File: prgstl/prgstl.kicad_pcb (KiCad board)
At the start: 2 copper layers, 76.2 x 50.8 mm, 49 parts, among them J2 STM32WORLD_BASE, Q1 S9013, U1 AMS1117-3.3``, U2 STM32F103CBTx, U3 SRV05-4, Y1 X_8MHZ

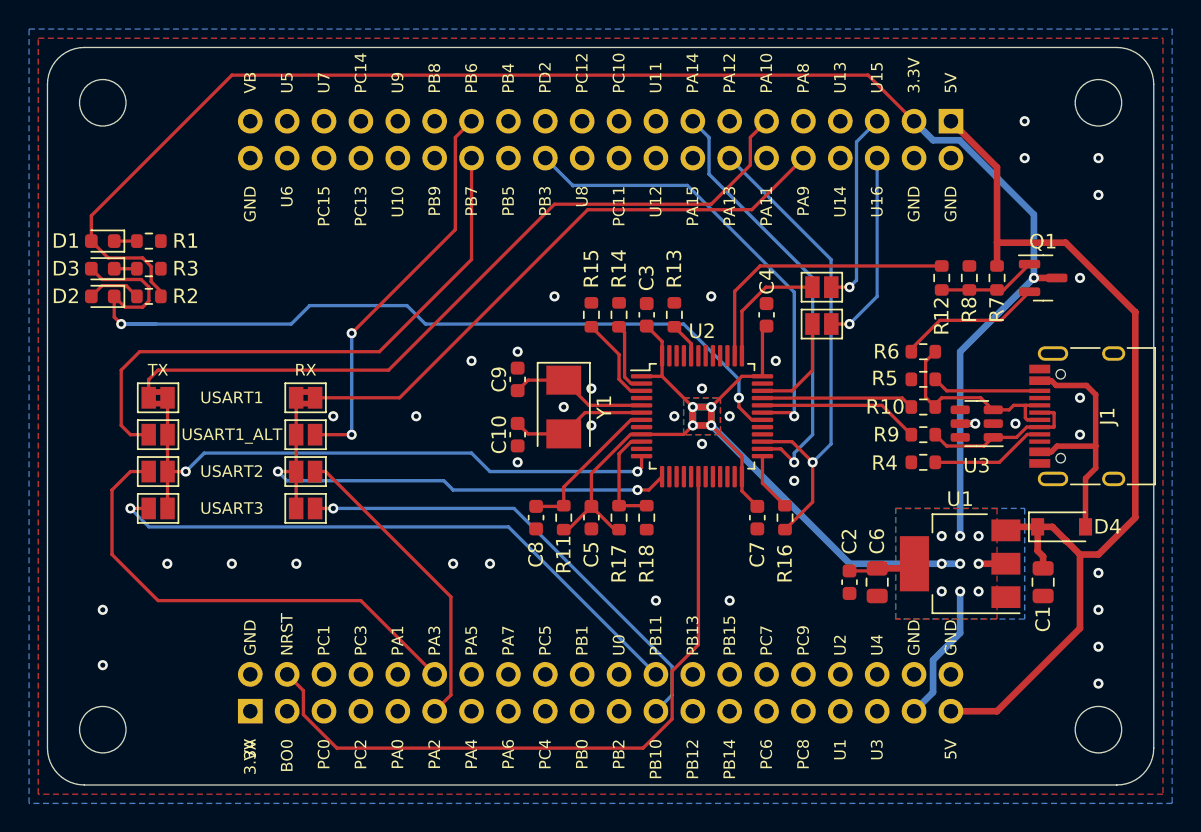
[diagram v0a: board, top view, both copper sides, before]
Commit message: Hmmmm
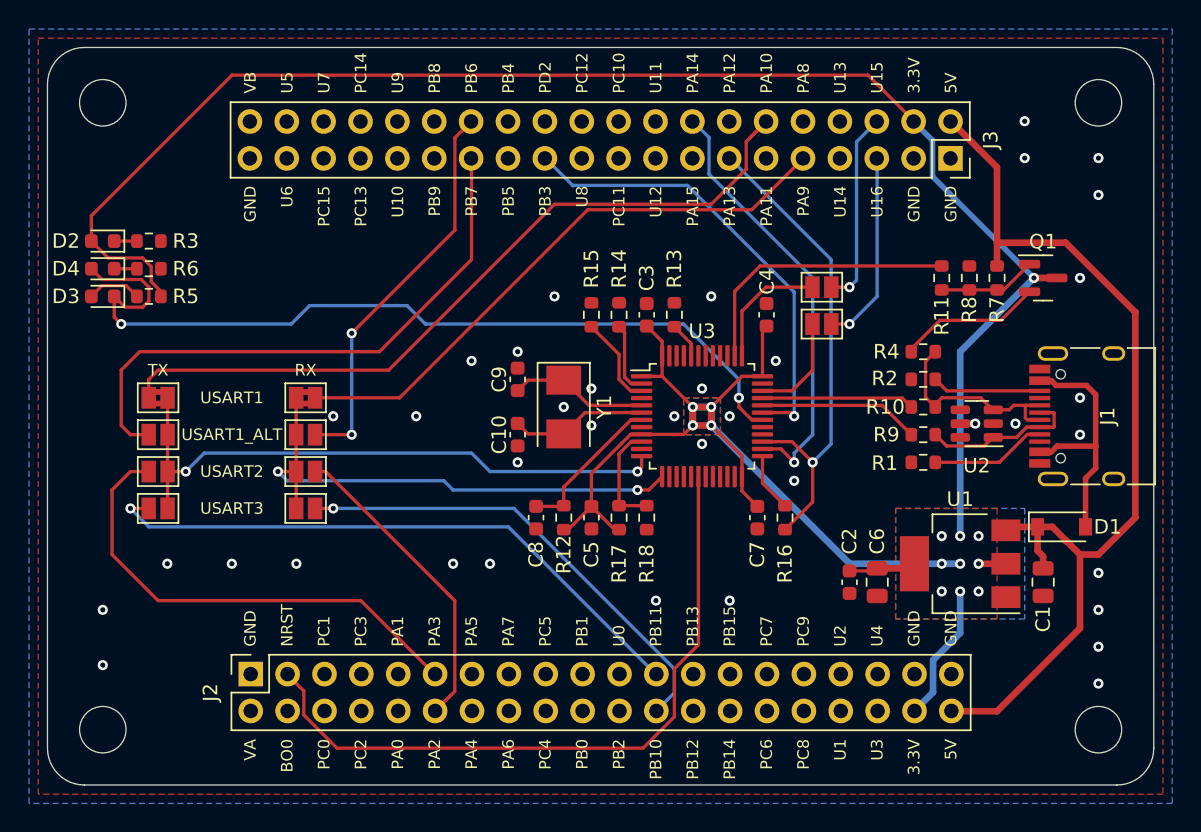
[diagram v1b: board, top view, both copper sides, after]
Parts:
- added J3: STM32WORLD_CONNECTOR_2, stm32world:PinSocket_2x20_P2.54mm_Vertical_Stackable, F.Cu at (176.5, 83.8)
- added J4: STM32WORLD_BOARD, stm32world:STM32WORLD_BOARD, F.Cu at (152.4, 101.6)
- J2: value STM32WORLD_BASE -> STM32WORLD_CONNECTOR_1; footprint stm32world:STM32WORLD_BASE -> stm32world:PinSocket_2x20_P2.54mm_Vertical_Stackable
- moved J2 29.9 mm to (128.3, 119.4), turned to 90 degrees
- renumbered D4 to D1, D1 to D2, D2 to D3, D3 to D4, R4 to R1, R12 to R11, R11 to R12, R5 to R2, R1 to R3, R6 to R4, R2 to R5, R3 to R6, U3 to U2, U2 to U3
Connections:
- J2 pad 1: unconnected-(J2-Pad1) -> GND
- J2 pad 11: USART2_TX -> USART2_RX
- J2 pad 12: USART2_RX -> USART2_TX
- J2 pad 2: GND -> unconnected-(J2-Pad2)
- J2 pad 23: USART3_TX -> USART3_RX
- J2 pad 24: USART3_RX -> USART3_TX
- J2 pad 3: unconnected-(J2-Pad3) -> T_RST
- J2 pad 37: +3V3 -> GND
- J2 pad 38: GND -> +3V3
- J2 pad 39: +5V -> GND
- J2 pad 4: T_RST -> unconnected-(J2-Pad4)
- J2 pad 40: GND -> +5V
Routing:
- net LED: track 61.9 -> 59.5 mm
- net USART2_TX: track 21.3 -> 23.3 mm
- net USART1_RX: track 52.3 -> 53.9 mm
- net +3V3: track 194.0 -> 192.9 mm

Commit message: Tweaking
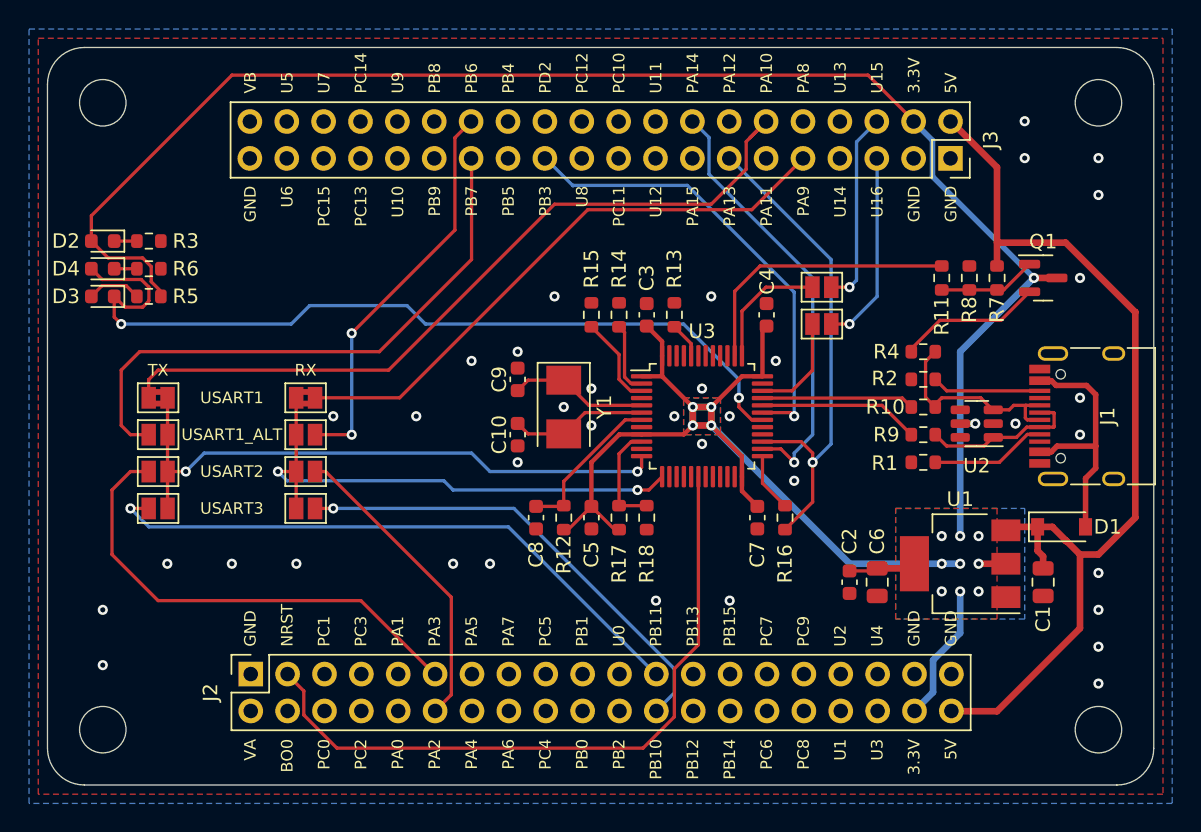
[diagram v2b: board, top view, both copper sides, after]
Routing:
- net USART2_TX: track 23.3 -> 21.3 mm
- net +3V3: track 192.9 -> 193.8 mm
